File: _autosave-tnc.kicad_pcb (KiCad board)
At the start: 2 copper layers, 56.6 x 31 mm, 55 parts, among them CON1 PJ2030D, K1 MK12C02, P1 CONN_3X2, P2 CONN_2, Q1 BC847C, SW1 SW_PUSH, U1 HC-05, U2 APE8800N, U3 BU33TD3WG, U4 ATMEGA328P-A, X1 CRYSTAL_SMD

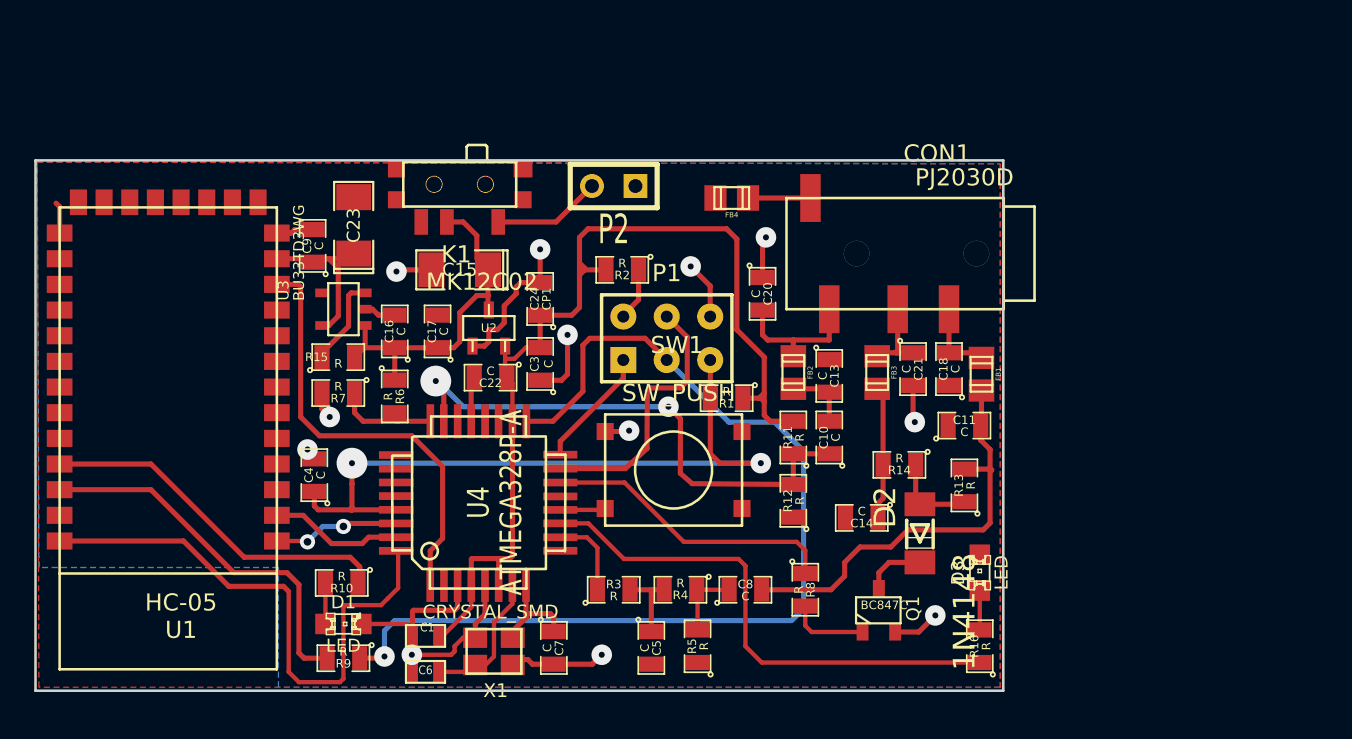
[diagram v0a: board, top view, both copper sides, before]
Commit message: Update gerber files and manufacture files
Signed-off-by: Angel Hitov <angelhitov@gmail.com>
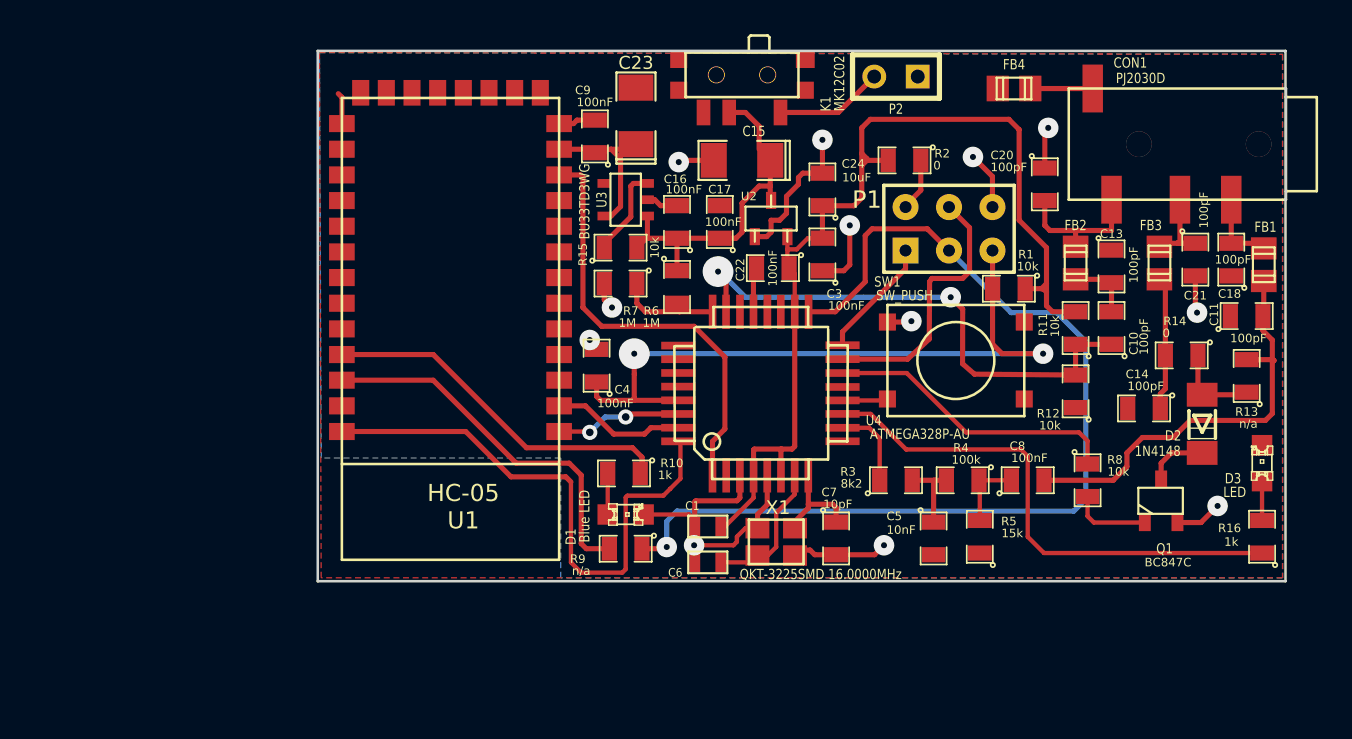
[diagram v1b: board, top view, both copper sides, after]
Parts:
- C1, C16, C17, C22, C23, C3, C4, C8, C9: value C -> 100nF
- C10, C11, C13, C14, C18, C20, C21: value C -> 100pF
- C15, C24: value CP1 -> 10uF
- C5: value C -> 10nF
- C6, C7: value C -> 10pF
- D1: value LED -> Blue LED
- FB1, FB2, FB3, FB4: value FILTER -> BLM21PG331SN1D
- P1: value CONN_3X2 -> ISP
- R1, R11, R12, R15, R8: value R -> 10k
- R10, R16: value R -> 1k
- R13, R9: value R -> n/a
- R14, R2: value R -> 0
- R3: value R -> 8k2
- R4: value R -> 100k
- R5: value R -> 15k
- R6, R7: value R -> 1M
- U4: value ATMEGA328P-A -> ATMEGA328P-AU
- X1: value CRYSTAL_SMD -> QKT-3225SMD 16.0000MHz
- moved C4 17.7 mm to (136.8, 103.0)
- moved C6 17.7 mm to (143.3, 114.5)
- moved U1 17.7 mm to (134.6, 88.8)
- moved C1 17.7 mm to (143.3, 112.4)
- moved C10 17.7 mm to (166.9, 100.8)
- moved C11 17.7 mm to (174.8, 100.1)
- moved C14 17.7 mm to (168.8, 105.5)
- moved C15 17.7 mm to (145.3, 91.0)
- moved C16 17.7 mm to (141.5, 94.6)
- moved C17 17.7 mm to (144.0, 94.6)
- moved C18 17.7 mm to (173.9, 96.8)
- moved C21 17.7 mm to (171.8, 96.8)
- moved C22 17.7 mm to (147.1, 97.3)
- moved C3 17.7 mm to (150.0, 96.5)
- moved C5 17.7 mm to (156.5, 113.1)
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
